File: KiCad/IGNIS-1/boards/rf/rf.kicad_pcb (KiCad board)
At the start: 2 copper layers, 7 parts, among them J30 SMA_antena, J42 Backplane_2x10, U30 RFM95W_SX1276_433MHz, U31 microSD

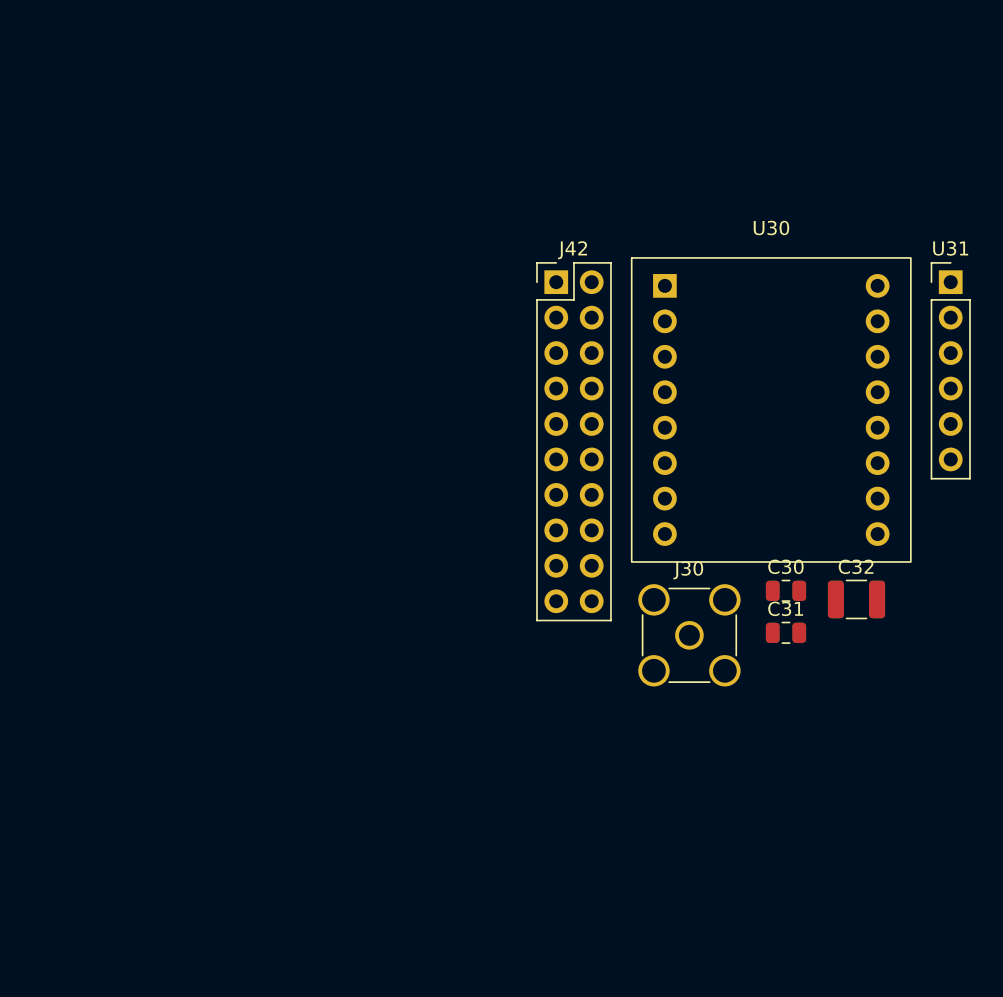
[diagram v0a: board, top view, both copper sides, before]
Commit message: Tracks listos en PCB
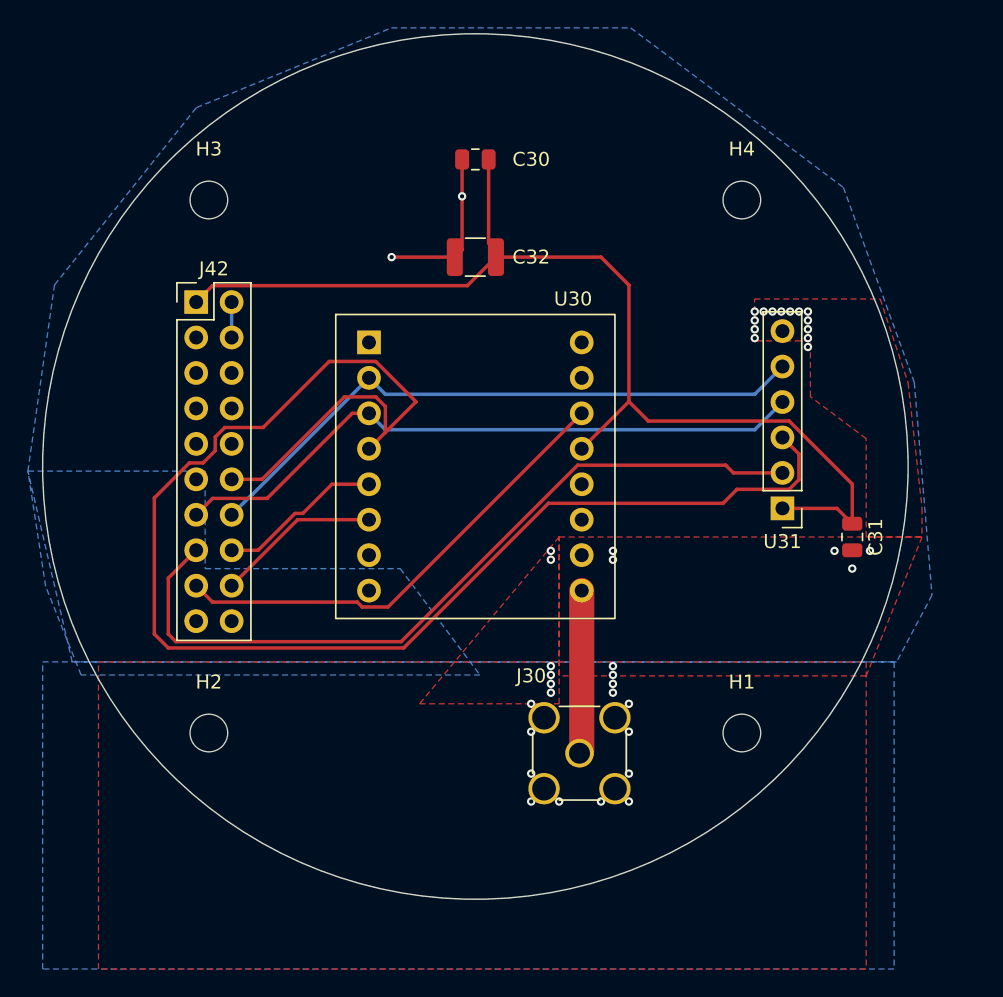
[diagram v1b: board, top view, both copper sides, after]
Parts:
- added H1: M2.5_hole, MountingHole:MountingHole_2.7mm_M2.5, F.Cu at (119.1, 119.1)
- added H2: M2.5_hole, MountingHole:MountingHole_2.7mm_M2.5, F.Cu at (80.9, 119.1)
- added H3: M2.5_hole, MountingHole:MountingHole_2.7mm_M2.5, F.Cu at (80.9, 80.9)
- added H4: M2.5_hole, MountingHole:MountingHole_2.7mm_M2.5, F.Cu at (119.1, 80.9)
- moved C30 38.1 mm to (100.0, 78.0), turned to 180 degrees
- moved C32 36.7 mm to (100.0, 85.0), turned to 180 degrees
- moved J42 25.8 mm to (80.0, 88.2)
- moved U30 21.6 mm to (100.0, 100.0)
- moved U31 20.2 mm to (122.0, 103.0), turned to 180 degrees
- moved J30 11.5 mm to (107.5, 120.5)
- moved C31 8.35 mm to (127.0, 105.0), turned to -90 degrees
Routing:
- net SCK: track 0.00 -> 109.8 mm
- net +3V3: track 0.00 -> 80.9 mm
- net CS_SD: track 0.00 -> 56.5 mm
- net MOSI: track 0.00 -> 46.3 mm
- net MISO: track 0.00 -> 44.8 mm
- net DIO0: track 0.00 -> 34.0 mm
- net GND: track 0.00 -> 15.5 mm, vias 0 -> 41
- net LORA_RST: track 0.00 -> 11.8 mm
- net NSS_LORA: track 0.00 -> 11.8 mm
- net /ANT: track 0.00 -> 11.7 mm
- added copper zone on B.Cu, net GND
- added copper zone on F.Cu, net GND
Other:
- board outline added: 62 x 62 mm
